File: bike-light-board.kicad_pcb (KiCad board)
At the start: 2 copper layers, 40.2 x 69 mm, 67 parts, among them J1 USB_Micro_MICRO_4P_DIP, J2 S2B-PH-SM4-TB, J3 AVR-ISP-6, P1 WirePad, P2 WirePad, P3 WirePad, P4 WirePad, Q1 NCE2003, Q2 NCE2003, Q3 NCE2003, Q4 SMD0805-20, SW1 SW_Push, U1 BRCL4054CME, U2 QMA7981, U3 SSP6206-33NR, U4 ATtiny84A-MU, U5 M74VHC1GT08DFT2G

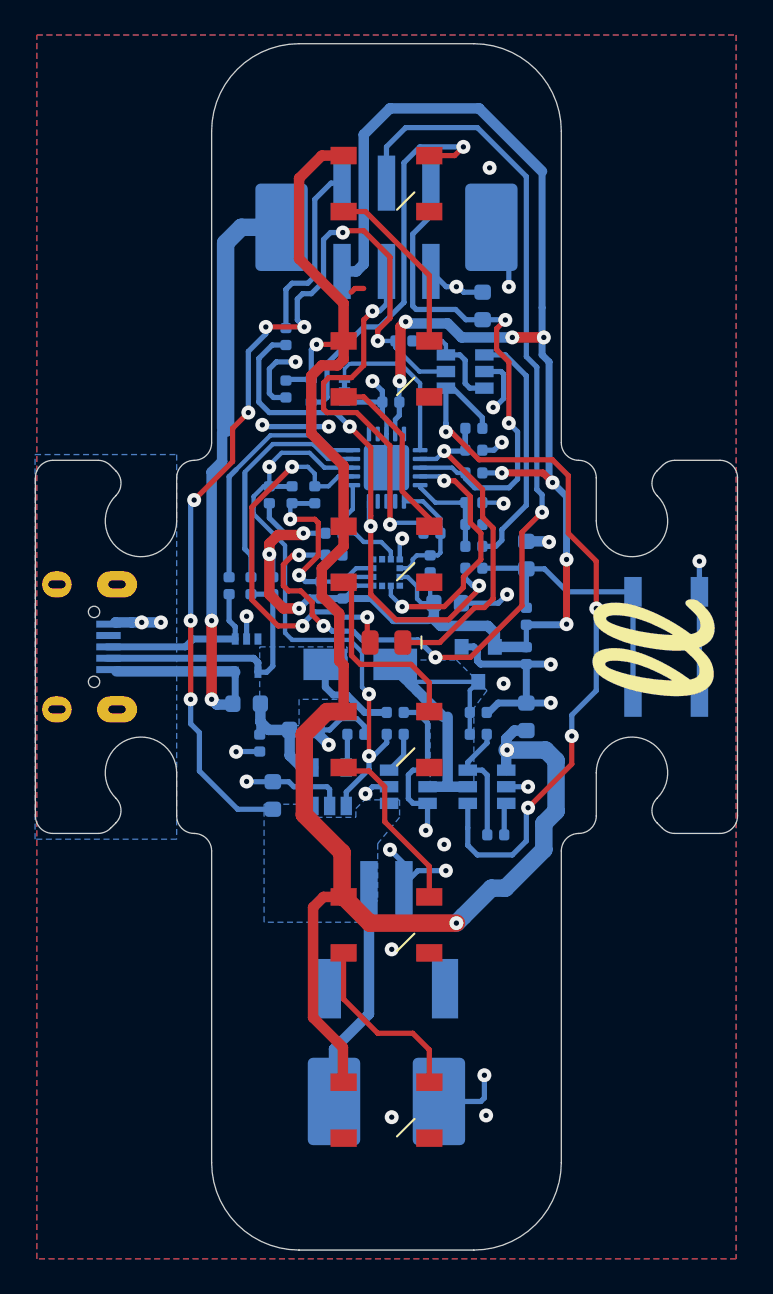
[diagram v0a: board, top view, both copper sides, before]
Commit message: update board
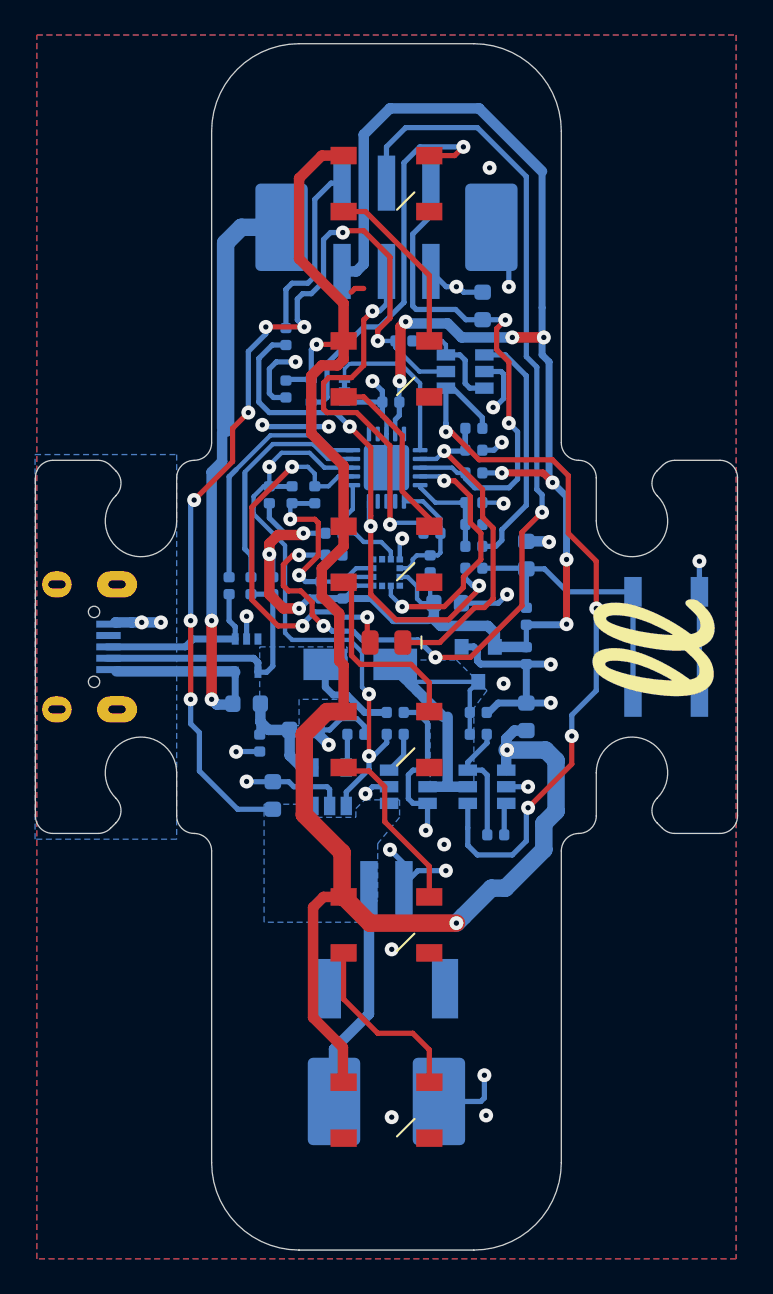
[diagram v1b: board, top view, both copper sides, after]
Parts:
- renumbered G*** to LG1, G*** to LG2, G*** to LG3
